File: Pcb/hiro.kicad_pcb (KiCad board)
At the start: 2 copper layers, 92.9 x 60.4 mm, 11 parts, among them J1 Micro_SD_Card_Det_Hirose_DM3AT, J2 AudioJack3, J3 Conn_01x09, U1 XIAO-ESP32-S3-Plus-SMD, U2 PCM5102A

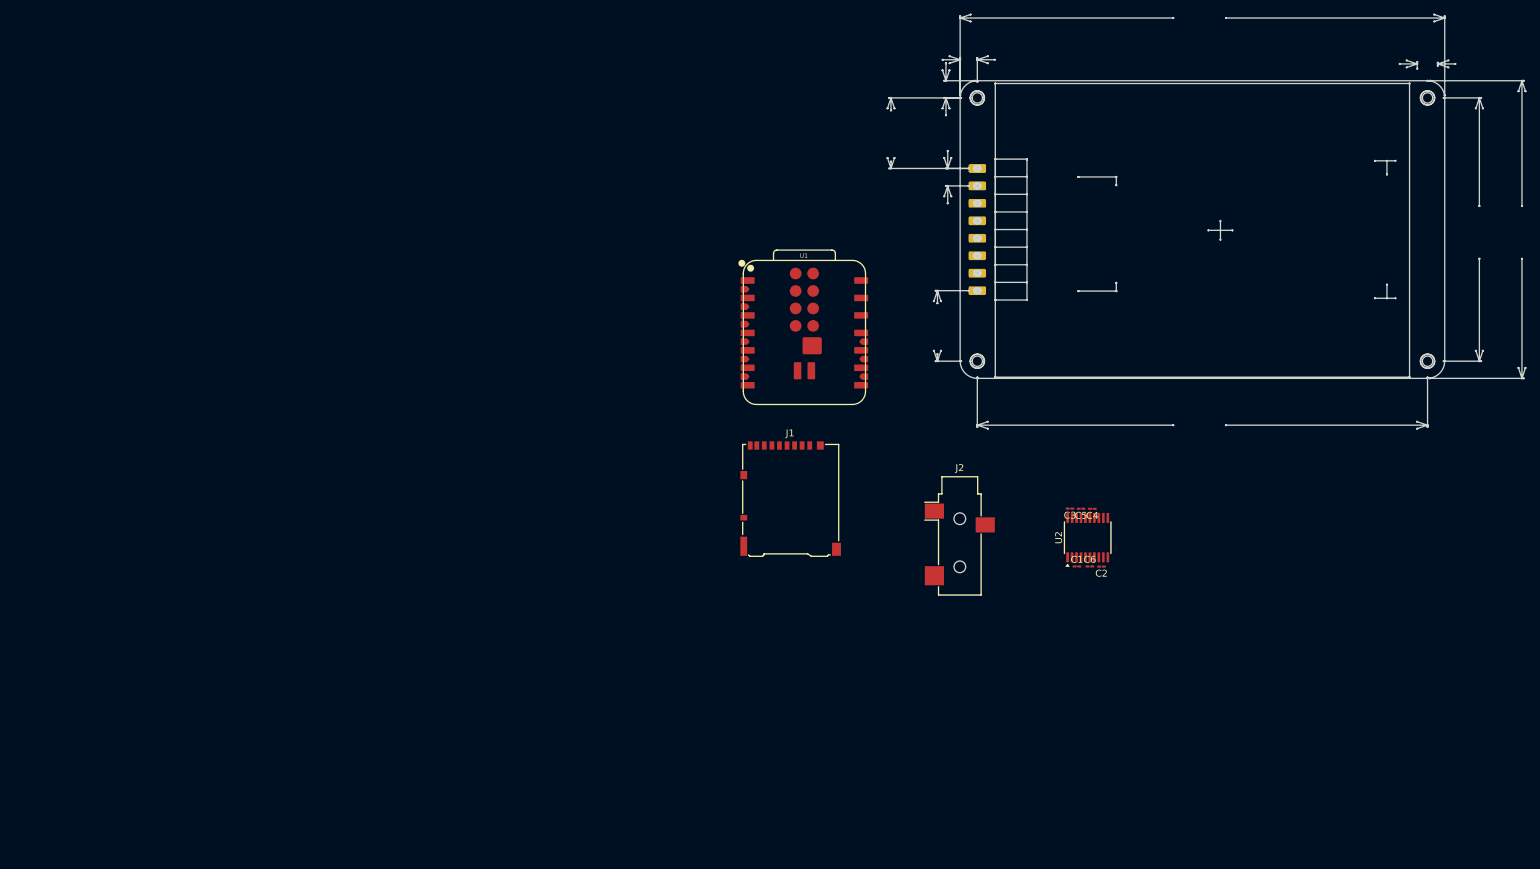
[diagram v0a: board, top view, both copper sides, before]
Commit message: THE OUTLINE WORKS YAYYY
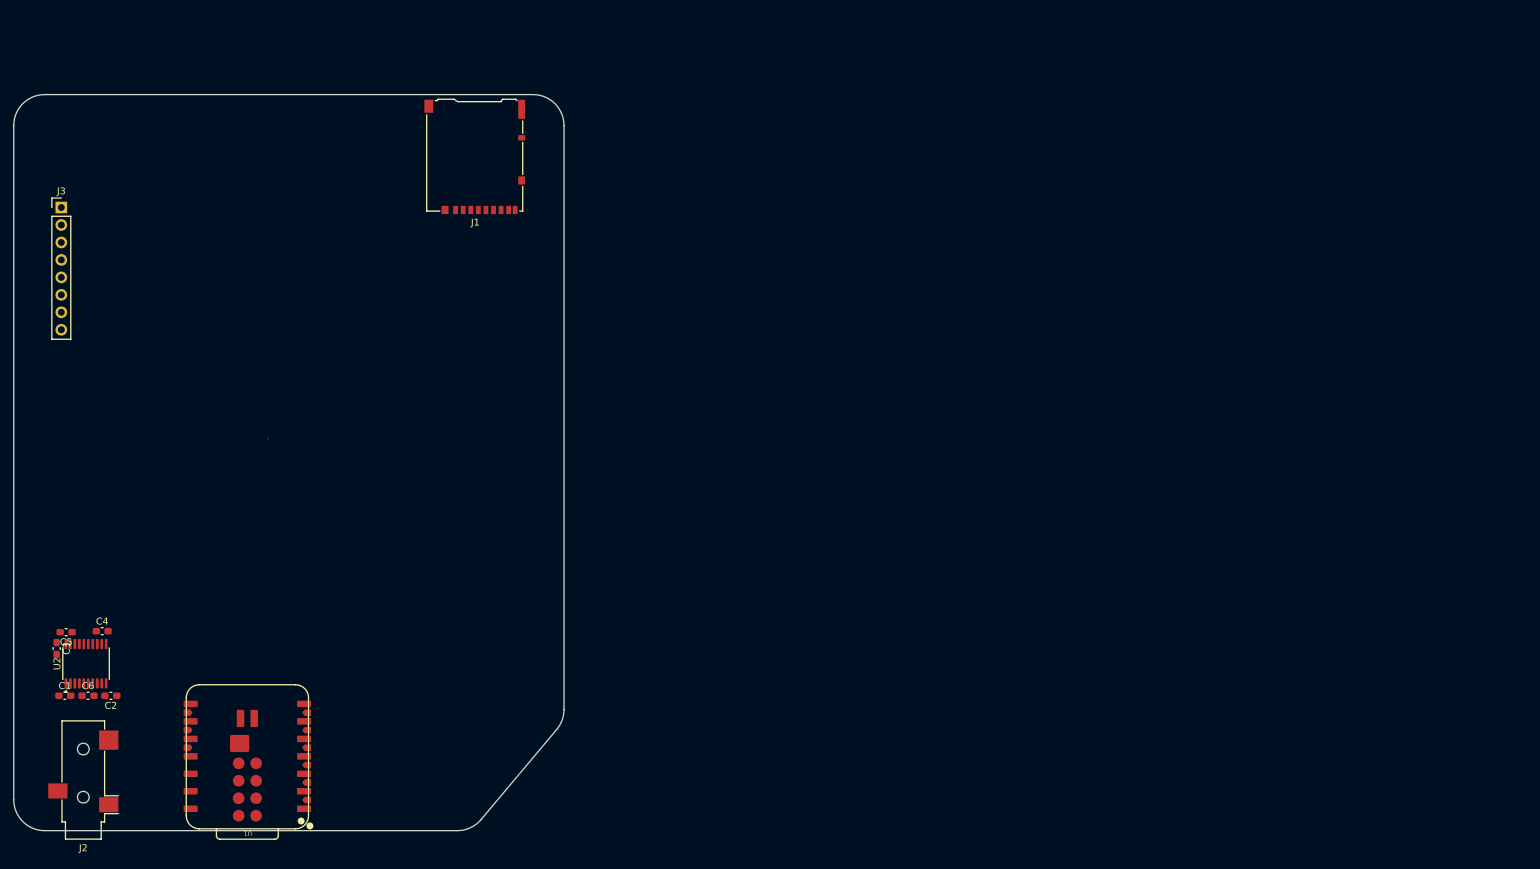
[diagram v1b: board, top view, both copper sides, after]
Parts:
- C1, C2, C3, C4, C5, C6: footprint Capacitor_SMD:C_01005_0402Metric_Pad0.57x0.30mm_HandSolder -> Capacitor_SMD:C_0603_1608Metric_Pad1.08x0.95mm_HandSolder
- J3: value Conn_01x09 -> Conn_01x08; footprint Libs:Waveshare 2.4_ lcd -> Connector_PinHeader_2.54mm:PinHeader_1x08_P2.54mm_Vertical
- moved J3 163.2 mm to (58.7, 50.0)
- moved C3 148.8 mm to (58.0, 114.2), turned to -90 degrees
- moved C5 148.7 mm to (59.4, 111.8)
- moved C1 148.4 mm to (59.2, 121.0)
- moved C6 147.0 mm to (62.5, 121.0)
- moved U2 146.9 mm to (62.2, 116.4)
- moved C2 145.3 mm to (65.9, 121.0)
- moved C4 145.1 mm to (64.6, 111.6), turned to 0 degrees
- moved J2 132.4 mm to (61.9, 133.3), turned to 180 degrees
- moved U1 101.8 mm to (85.7, 129.8), turned to -90 degrees
- moved J1 67.7 mm to (118.8, 42.6), turned to 180 degrees
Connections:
- J3 pad 1: unconnected-(J3-Pin_1-Pad1) -> +3.3V
- J3 pad 2: unconnected-(J3-Pin_2-Pad2) -> GND
- J3 pad 3: unconnected-(J3-Pin_3-Pad3) -> /DIN
- J3 pad 4: unconnected-(J3-Pin_4-Pad4) -> /CLK
- J3 pad 5: unconnected-(J3-Pin_6-Pad6) -> /CS
- J3 pad 6: unconnected-(J3-Pin_7-Pad7) -> /DC
- J3 pad 7: unconnected-(J3-Pin_8-Pad8) -> /RST
- J3 pad 8: Net-(J3-Pin_9) -> /BL
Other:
- board size 92.9 x 60.4 mm -> 80.1 x 107.1 mm
